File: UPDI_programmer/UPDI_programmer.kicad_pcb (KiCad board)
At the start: 2 copper layers, 67.3 x 25.4 mm, 32 parts, among them J1 UPDI, J2 ICSP, J3 USB_B, U1 FT230XS, U2 ATmega168P-20AU, Y1 16MHz

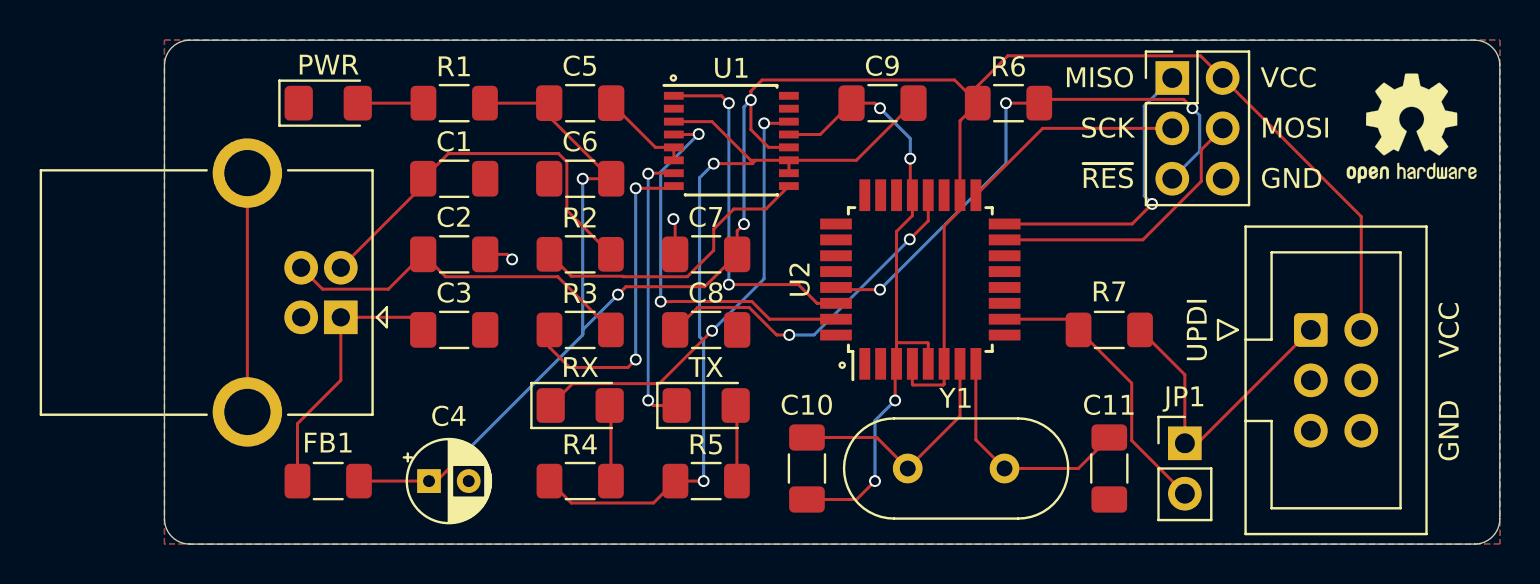
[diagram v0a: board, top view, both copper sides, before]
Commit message: PCB RC2
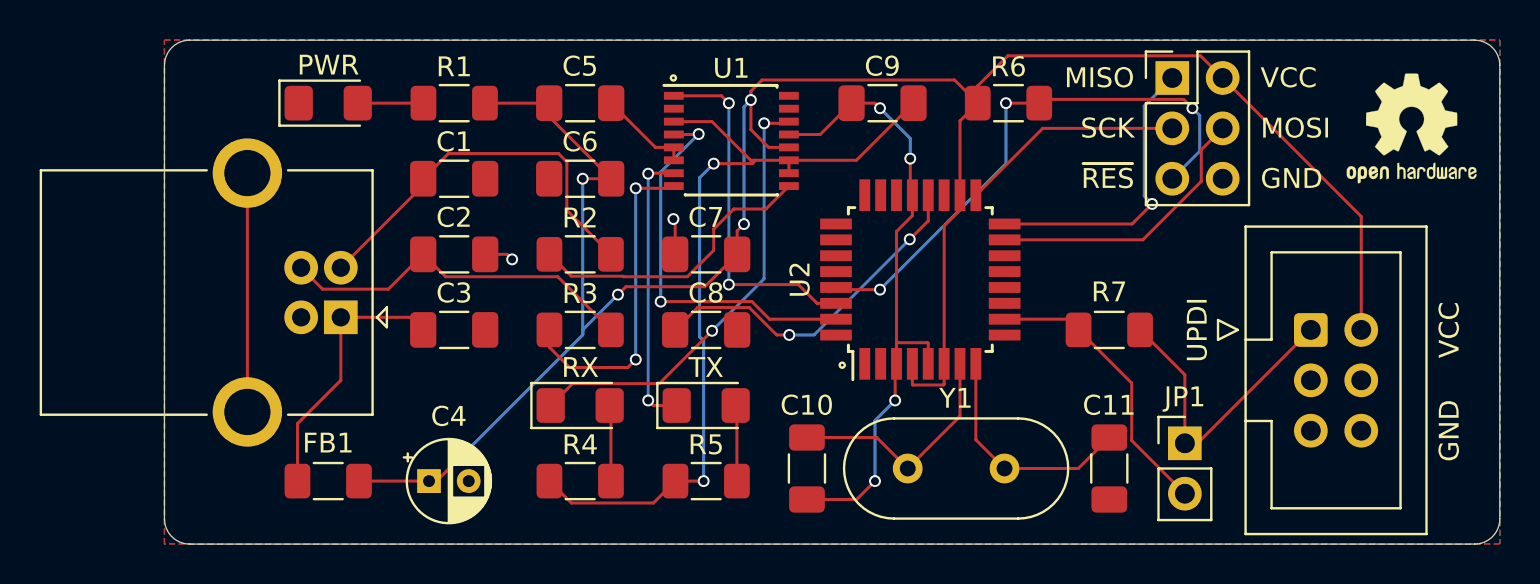
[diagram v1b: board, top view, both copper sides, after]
